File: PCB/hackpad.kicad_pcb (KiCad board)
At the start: 2 copper layers, 80.3 x 41.5 mm, 11 parts, among them J1 Conn_01x04_Pin, SW1 SW_Push, SW2 SW_Push, SW3 SW_Push, SW4 SW_Push, SW5 RotaryEncoder_Switch, U1 XIAO-RP2040-DIP

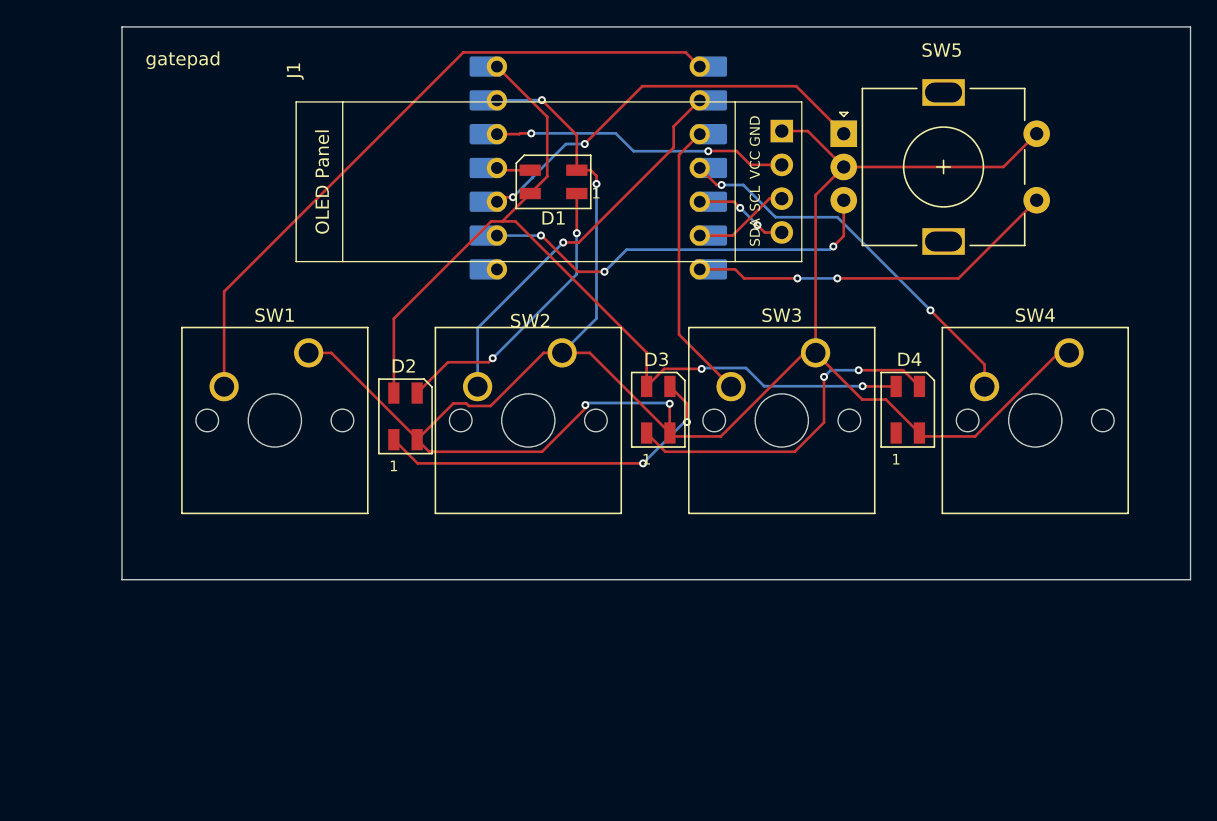
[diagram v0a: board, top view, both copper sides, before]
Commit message: updates from the last 4 days
mostly 3d models for cad stuff and kicad mod..?
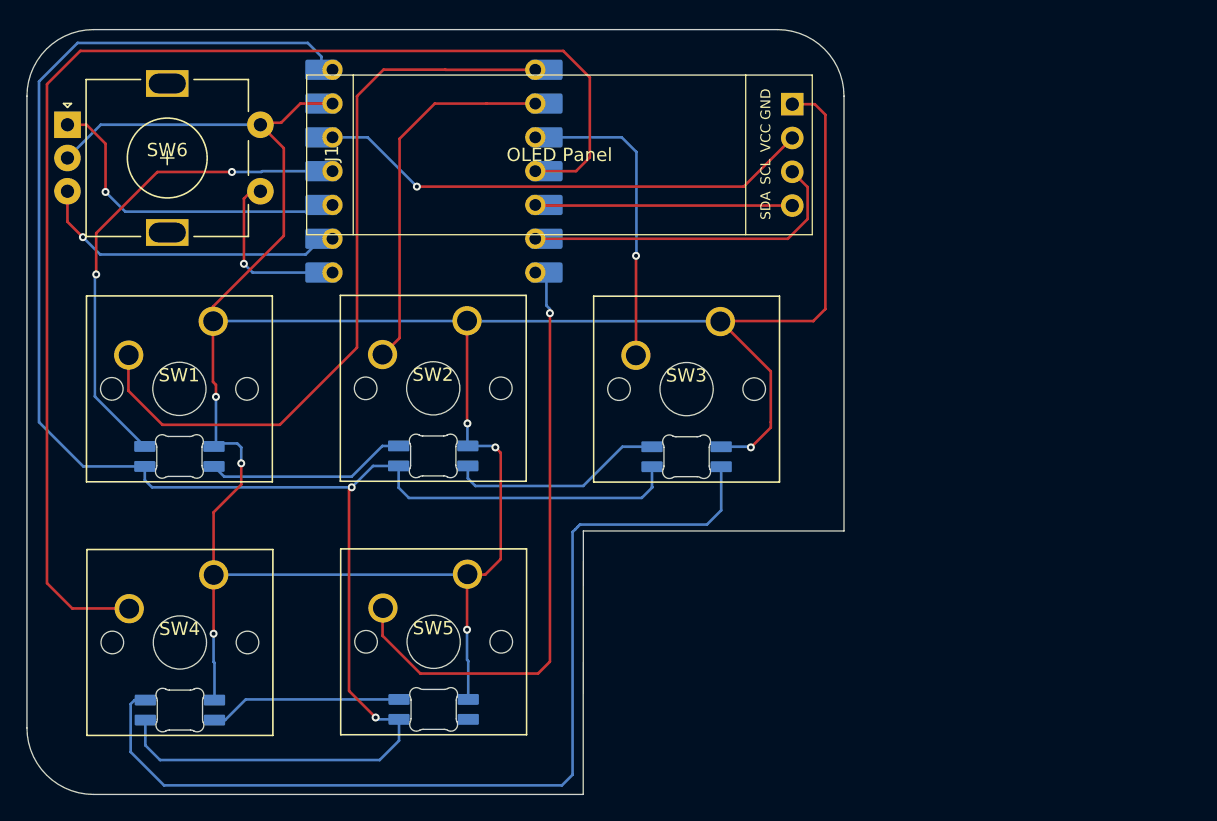
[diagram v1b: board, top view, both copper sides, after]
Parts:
- added D5: SK6812MINI, Custom:MX_SK6812MINI-E_REV(1), F.Cu at (173.9, 83.3)
- added G***: LOGO, LOGO, B.Cu at (164.3, 73.1)
- added G***: LOGO, LOGO, B.Cu at (193.8, 45.3)
- added G***: LOGO, LOGO, B.Cu at (194.4, 64.5)
- added SW6: RotaryEncoder_Switch, Custom:Rotary_EncoderRotaryEncoder_Alps_EC11E-Switch_Vertical_H20mm_custom, F.Cu at (153.8, 46.9)
- D1, D2, D3, D4: footprint LED_SMD:LED_SK6812MINI_PLCC4_3.5x3.5mm_P1.75mm -> Custom:MX_SK6812MINI-E_REV(1)
- SW1, SW2, SW3, SW4: footprint Button_Switch_Keyboard:SW_Cherry_MX_1.00u_PCB -> Custom:cherry_mx_1.00u_pcb_custom
- SW5: value RotaryEncoder_Switch -> SW_Push; footprint Rotary_Encoder:RotaryEncoder_Alps_EC11E-Switch_Vertical_H20mm -> Custom:cherry_mx_1.00u_pcb_custom
- moved SW4 70.3 mm to (154.8, 83.3)
- moved D4 57.4 mm to (154.8, 83.4), turned to 0 degrees
- moved SW5 49.1 mm to (173.8, 83.3)
- moved D1 32.1 mm to (154.8, 64.3), turned to 0 degrees
- moved U1 12.4 mm to (173.9, 47.9)
- moved SW1 10.1 mm to (154.7, 64.3)
- moved SW3 10.1 mm to (192.8, 64.3)
- moved SW2 10.1 mm to (173.8, 64.2)
- moved D2 2.97 mm to (173.8, 64.3), turned to 0 degrees
- moved D3 2.63 mm to (192.9, 64.3), turned to 0 degrees
- moved J1 2.17 mm to (164.3, 40.7)
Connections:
- D4 pad 1: unconnected-(D4-DOUT-Pad1) -> Net-(D4-DOUT)
- U1 pad 8: unconnected-(U1-GPIO1/RX-Pad8)_1 -> Button 6
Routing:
- net +5V: track 68.8 -> 146.4 mm
- net Button 4: track 29.2 -> 97.7 mm, vias 2 -> 0
- net Net-(D3-DOUT): track 26.1 -> 72.8 mm, vias 2 -> 0
- net GND: track 158.3 -> 201.0 mm, vias 4 -> 7
- net LED Data: track 2.57 -> 36.5 mm, vias 0 -> 2
- net OLED SCL: track 7.31 -> 25.1 mm
- net Button 5: track 28.0 -> 45.5 mm, vias 2 -> 1
- net +3.3V: track 22.4 -> 37.6 mm, vias 2 -> 1
- net Net-(D4-DOUT): track 0.00 -> 14.5 mm
- net Button 6: track 0.00 -> 12.9 mm, vias 0 -> 1
- net OLED SDA: track 7.12 -> 19.3 mm, vias 2 -> 0
- net Net-(D2-DOUT): track 27.3 -> 16.2 mm, vias 2 -> 0
- net Encoder B: track 31.0 -> 22.9 mm, vias 3 -> 1
- net Encoder A: track 31.2 -> 24.1 mm, vias 2 -> 1
- net Net-(D1-DOUT): track 21.8 -> 15.2 mm, vias 2 -> 0
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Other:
- board size 80.3 x 41.5 mm -> 61.4 x 57.5 mm
- board text added: "Feat. Heidi, turtle, shark, quokka, cat, sheep, crab, nigersaurus, Orpheus"
- board text added: "XIAO HERE"
- board text added: "jigu's toastpad"
- board text removed: "Xiao here!"
- board text removed: "gatepad"
